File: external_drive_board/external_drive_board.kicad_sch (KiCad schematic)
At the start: 31 parts, among them J1 MD-90SM, J2 MD-90SM, J3 Conn_02x17_Odd_Even, J4 Conn_01x04, J5 Conn_01x02, J6 Conn_01x02, J7 Conn_01x02, SW1 SW_DIP_x04, U1 74LS125, U2 74LS85, U3 74LS595, U4 74LS165, U5 74LS04, U6 74LS165

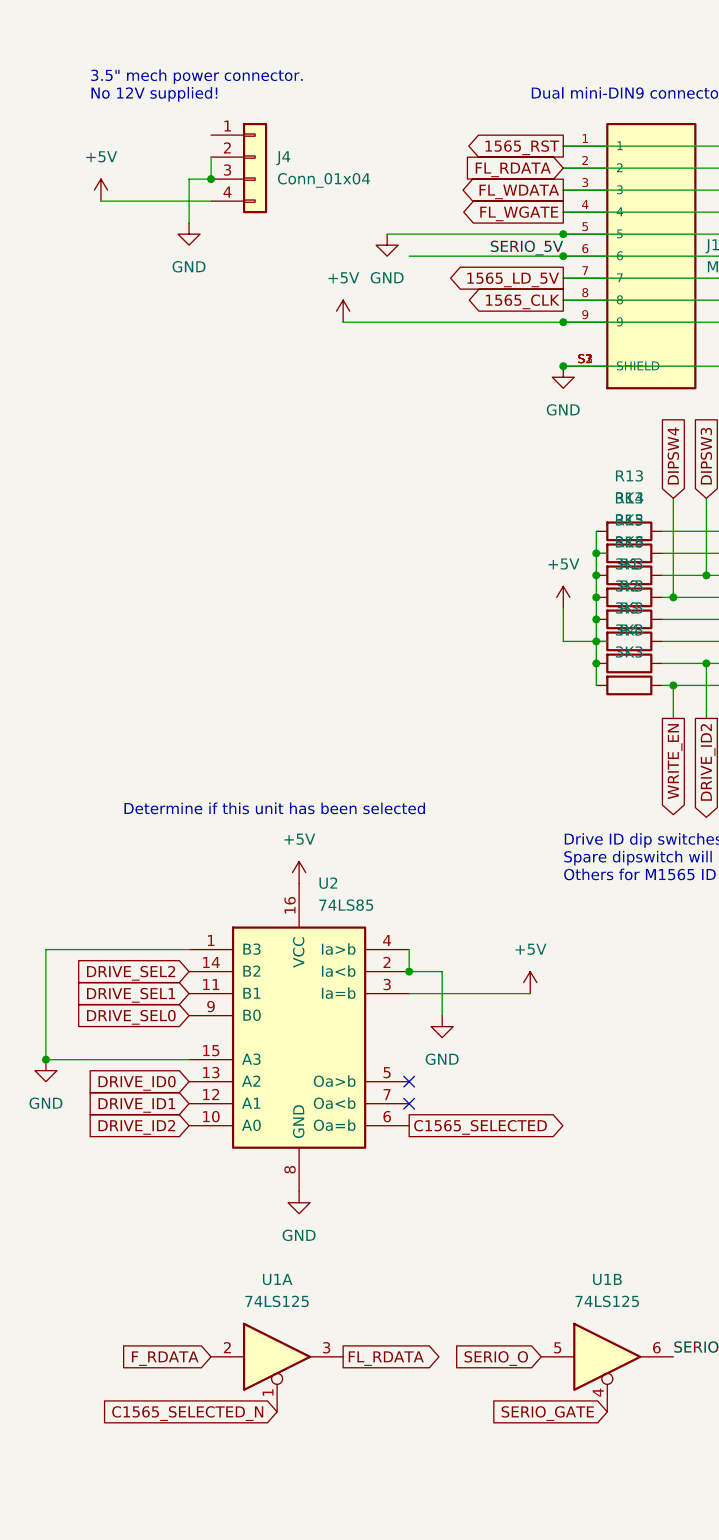
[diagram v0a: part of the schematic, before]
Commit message: more routing
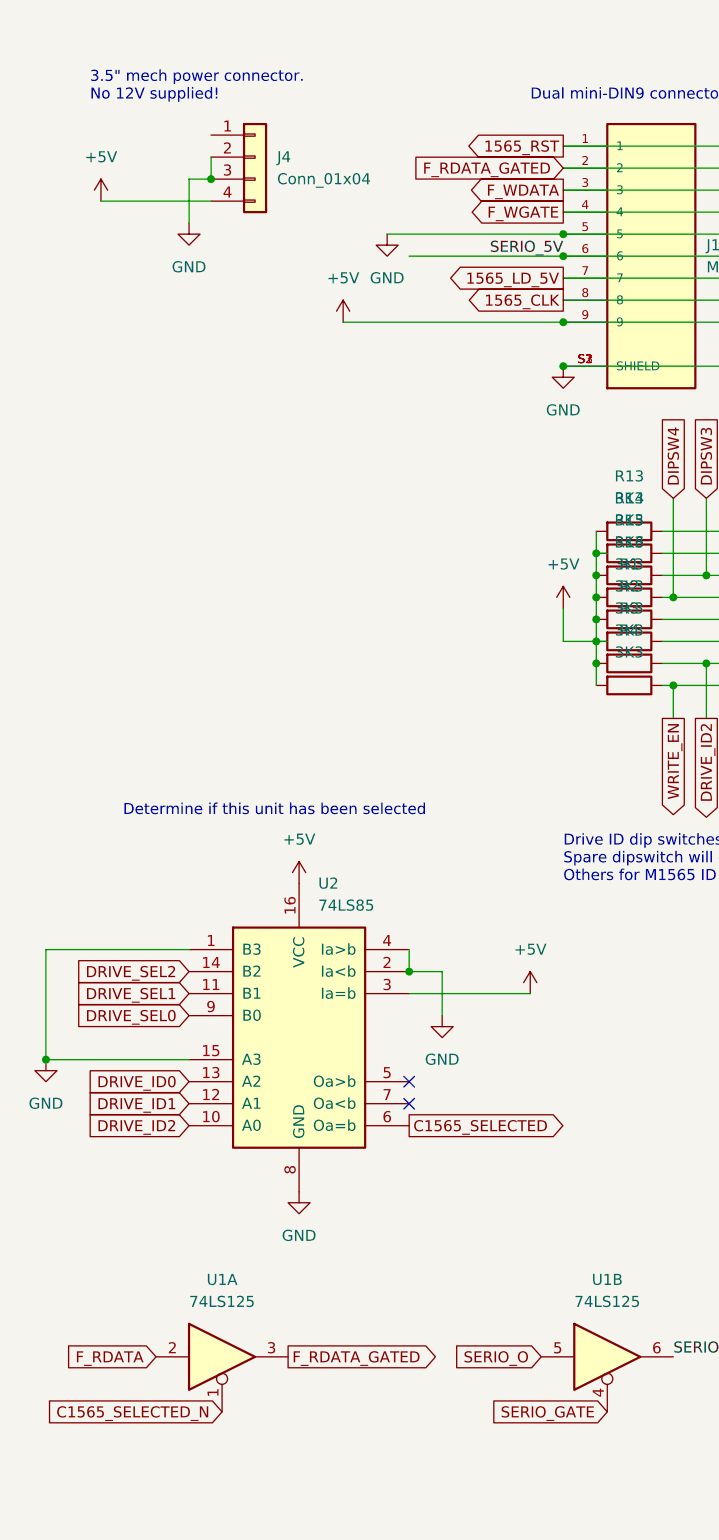
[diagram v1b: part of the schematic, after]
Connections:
- net FL_WDATA is gone; now on net F_WDATA: J1.3, J2.3
- net FL_WGATE is gone; now on net F_WGATE: J1.4, J2.4
- net FL_RDATA renamed F_RDATA_GATED
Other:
- moved on the sheet: U1A
